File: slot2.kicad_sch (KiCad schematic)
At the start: 1 part

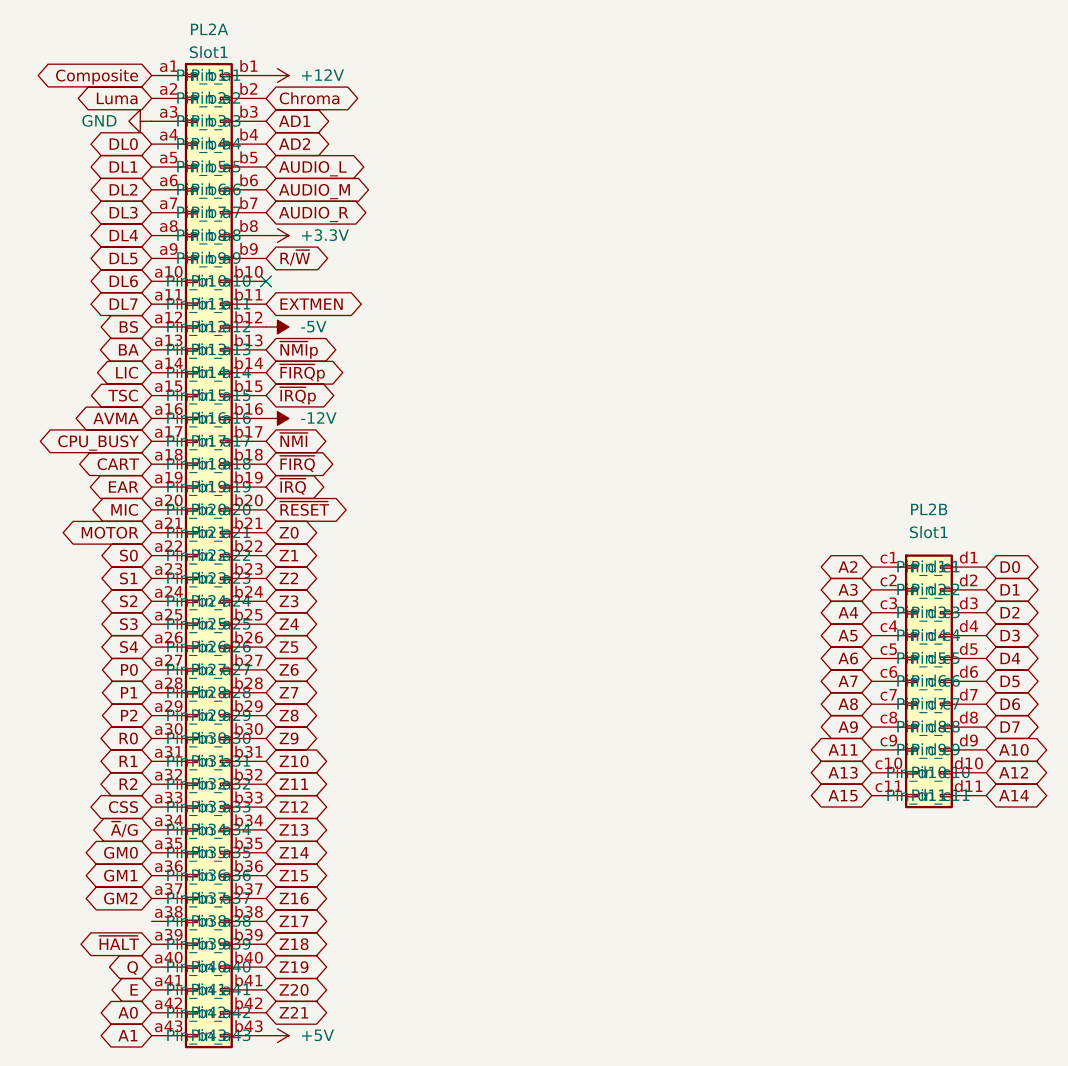
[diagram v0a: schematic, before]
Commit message: board layout
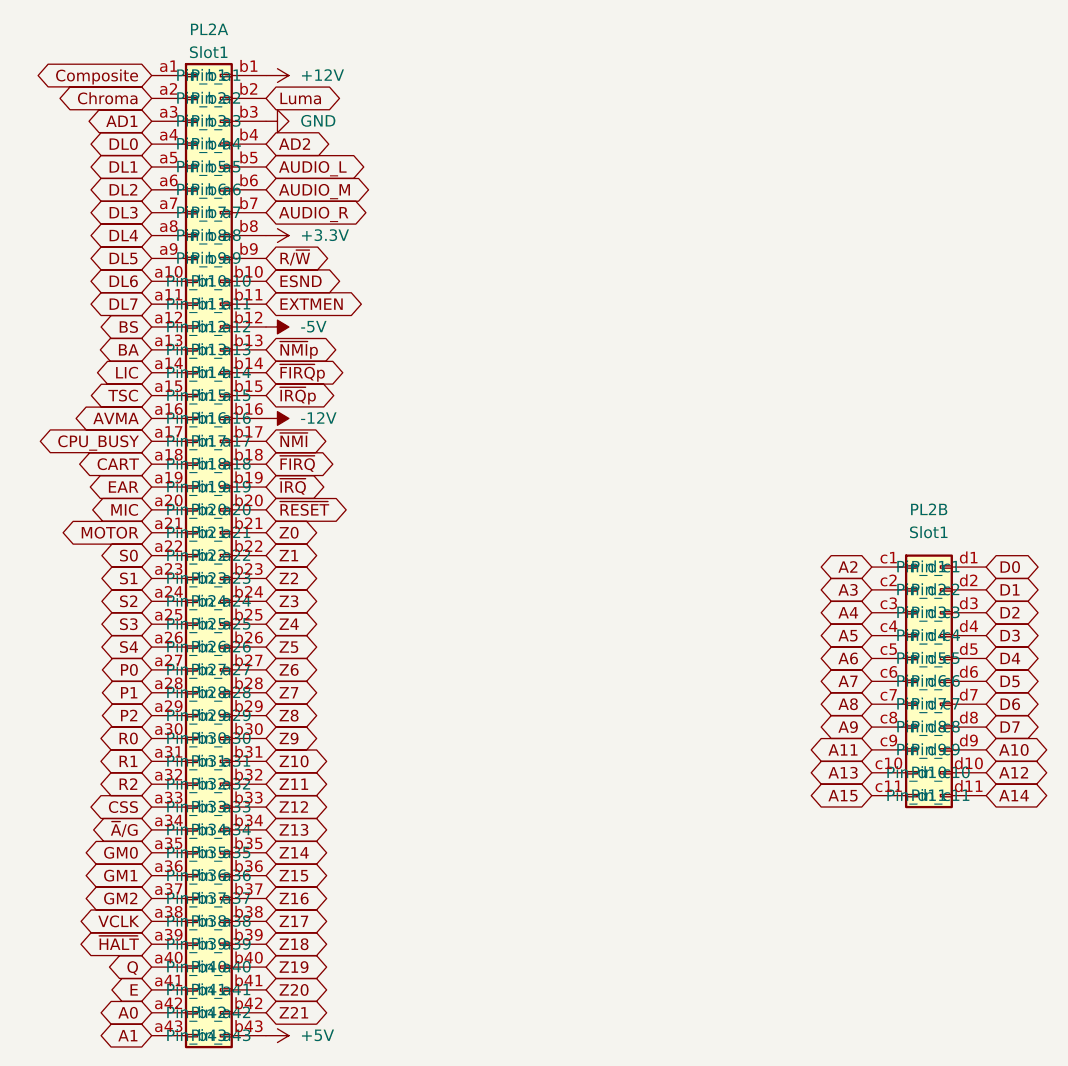
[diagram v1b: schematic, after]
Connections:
- net AD1: now also PL2.a3 (Pin_a3); no longer PL2.b3 (Pin_b3)
- net Chroma: now also PL2.a2 (Pin_a2); no longer PL2.b2 (Pin_b2)
- net GND: now also PL2.b3 (Pin_b3); no longer PL2.a3 (Pin_a3)
- net Luma: now also PL2.b2 (Pin_b2); no longer PL2.a2 (Pin_a2)
- net VCLK: now reaches PL2.a38 (Pin_a38)
- net ESND: now reaches PL2.b10 (Pin_b10)
- no-connect marks 1 -> 0
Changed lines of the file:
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@@
 	(generator_version "8.0")
 	(paper "A4")
-	(no_connect
-		(at 114.3 74.93)
-	)
 	(global_label "AD1"
 		(shape bidirectional)
-		(at 114.3 57.15 0)
+		(at 101.6 57.15 180)
 		(fields_autoplaced yes)
 		(effects
@@
 				(size 1.27 1.27)
 			)
-			(justify left)
+			(justify right)
 		)
 		(property "Intersheetrefs" "${INTERSHEET_REFS}"
-			(at 121.9646 57.15 0)
+			(at 93.9354 57.15 0)
 			(effects
 				(font
 					(size 1.27 1.27)
 				)
-				(justify left)
+				(justify right)
 				(hide yes)
 			)
@@
 	(global_label "Luma"
 		(shape bidirectional)
-		(at 101.6 54.61 180)
+		(at 114.3 54.61 0)
 		(fields_autoplaced yes)
 		(effects
@@
 				(size 1.27 1.27)
 			)
-			(justify right)
+			(justify left)
 		)
 		(property "Intersheetrefs" "${INTERSHEET_REFS}"
-			(at 92.4841 54.61 0)
+			(at 123.4159 54.61 0)
 			(effects
 				(font
 					(size 1.27 1.27)
 				)
-				(justify right)
+				(justify left)
 				(hide yes)
 			)
@@
 		)
 	)
+	(global_label "VCLK"
+		(shape bidirectional)
+		(at 101.6 146.05 180)
+		(fields_autoplaced yes)
+		(effects
+			(font
+				(size 1.27 1.27)
+			)
+			(justify right)
+		)
+		(property "Intersheetrefs" "${INTERSHEET_REFS}"
+			(at 92.8468 146.05 0)
+			(effects
+				(font
+					(size 1.27 1.27)
+				)
+				(justify right)
+				(hide yes)
+			)
+		)
+	)
 	(global_label "A14"
 		(shape bidirectional)
@@
 	(global_label "Chroma"
 		(shape bidirectional)
-		(at 114.3 54.61 0)
+		(at 101.6 54.61 180)
 		(fields_autoplaced yes)
 		(effects
@@
 				(size 1.27 1.27)
 			)
-			(justify left)
+			(justify right)
 		)
 		(property "Intersheetrefs" "${INTERSHEET_REFS}"
-			(at 125.593 54.61 0)
+			(at 90.307 54.61 0)
 			(effects
 				(font
 					(size 1.27 1.27)
 				)
-				(justify left)
+				(justify right)
 				(hide yes)
 			)
@@
 		)
 	)
+	(global_label "ESND"
+		(shape bidirectional)
+		(at 114.3 74.93 0)
+		(fields_autoplaced yes)
+		(effects
+			(font
+				(size 1.27 1.27)
+			)
+			(justify left)
+		)
+		(property "Intersheetrefs" "${INTERSHEET_REFS}"
+			(at 122.2442 74.93 0)
+			(effects
+				(font
+					(size 1.27 1.27)
+				)
+				(justify left)
+				(hide yes)
+			)
+		)
+	)
 	(global_label "R2"
 		(shape bidirectional)
@@
 	(symbol
 		(lib_id "power:GND")
-		(at 101.6 57.15 270)
+		(at 114.3 57.15 90)
+		(mirror x)
 		(unit 1)
 		(exclude_from_sim no)
@@
 		(fields_autoplaced yes)
 		(property "Reference" "#PWR05"
-			(at 95.25 57.15 0)
+			(at 120.65 57.15 0)
 			(effects
 				(font
@@
 		)
 		(property "Value" "GND"
-			(at 97.79 57.1499 90)
+			(at 118.11 57.1499 90)
 			(effects
 				(font
@@
 		)
 		(property "Footprint" ""
-			(at 101.6 57.15 0)
+			(at 114.3 57.15 0)
 			(effects
 				(font
@@
 		)
 		(property "Datasheet" ""
-			(at 101.6 57.15 0)
+			(at 114.3 57.15 0)
 			(effects
 				(font
@@
 		)
 		(property "Description" "Power symbol creates a global label with name \"GND\" , ground"
-			(at 101.6 57.15 0)
+			(at 114.3 57.15 0)
 			(effects
 				(font
